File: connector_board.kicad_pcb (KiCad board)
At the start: 2 copper layers, 40 x 22.5 mm, 2 parts, among them J1 Screw Terminal Block 5.00 mm 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

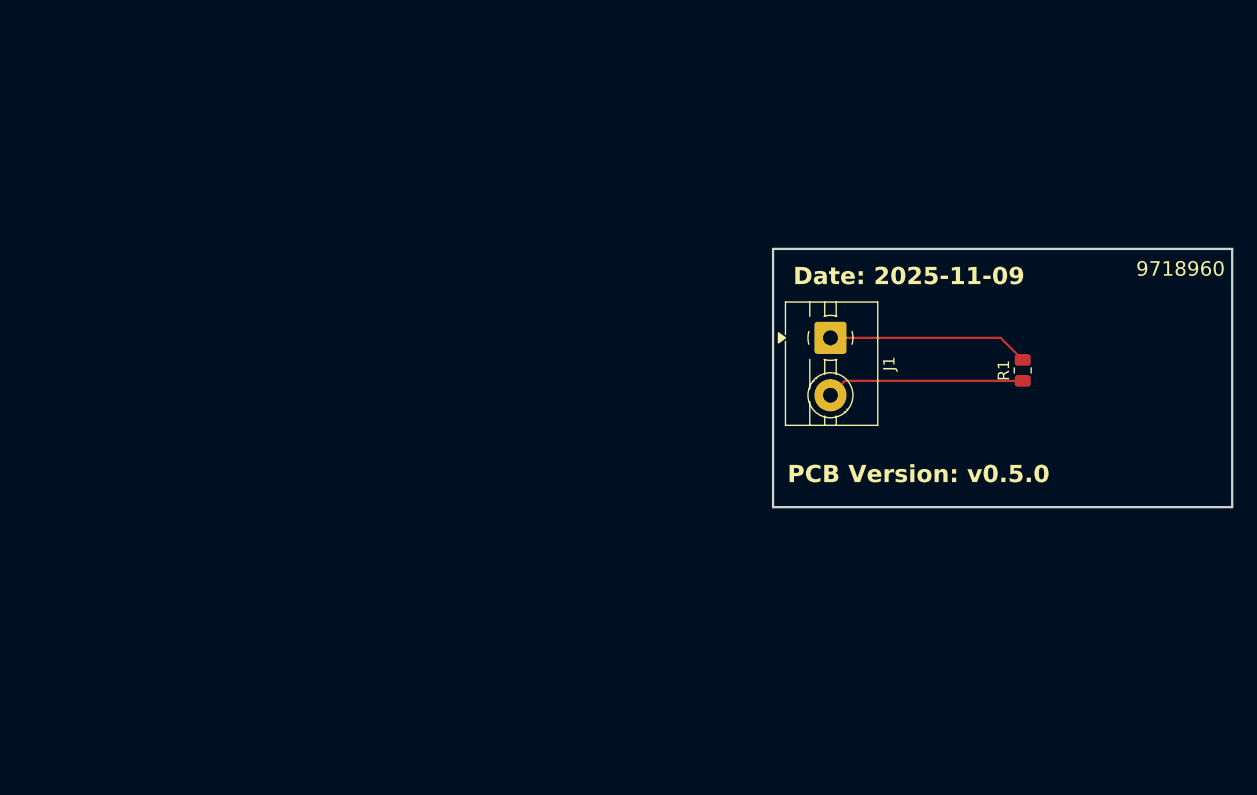
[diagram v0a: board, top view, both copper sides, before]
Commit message: feat: add connectors
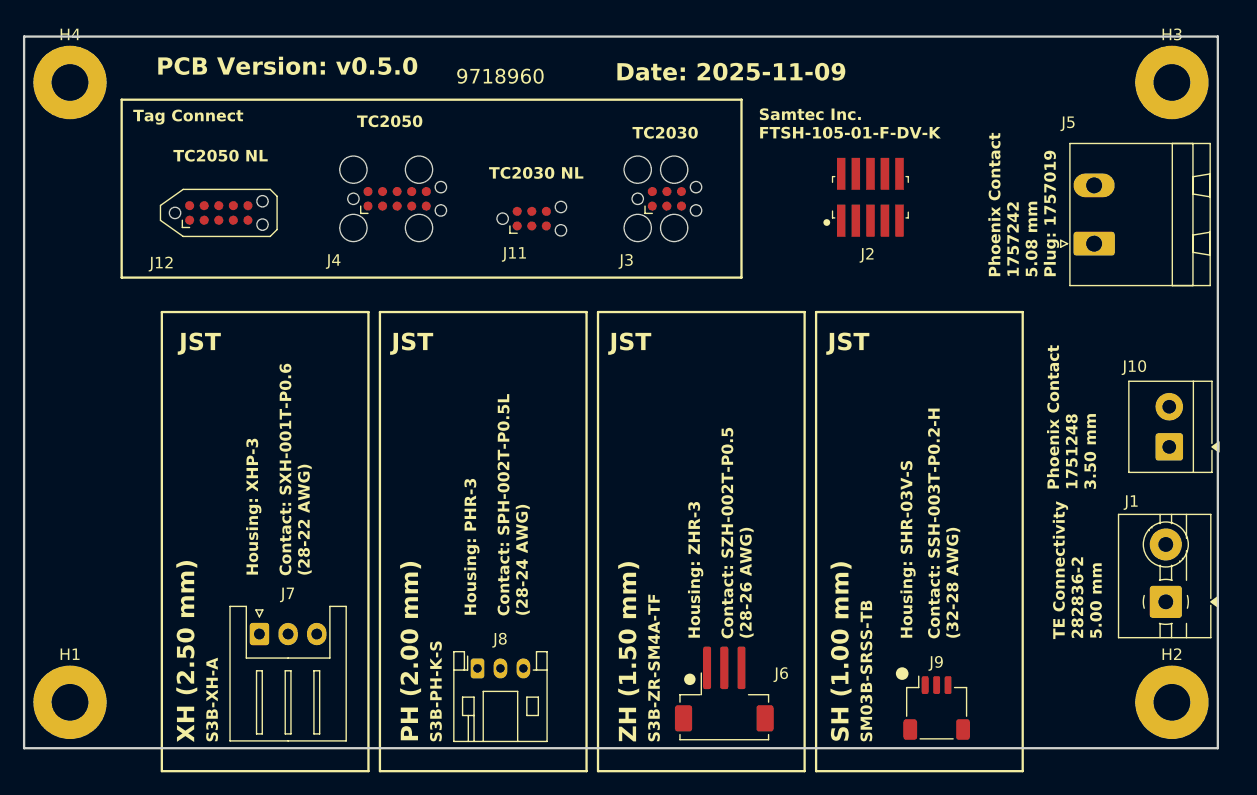
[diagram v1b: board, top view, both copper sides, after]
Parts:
- removed R1: 47k_0805, Resistor_SMD:R_0805_2012Metric
- added H1: MountingHole, MountingHole:MountingHole_3.2mm_M3_Pad, F.Cu at (78.0, 91.0)
- added H2: MountingHole, MountingHole:MountingHole_3.2mm_M3_Pad, F.Cu at (174.0, 91.0)
- added H3: MountingHole, MountingHole:MountingHole_3.2mm_M3_Pad, F.Cu at (174.0, 37.0)
- added H4: MountingHole, MountingHole:MountingHole_3.2mm_M3_Pad, F.Cu at (78.0, 37.0)
- added J10: Screw Terminal Block 3.50 mm 2 pol, 2s_connectors:TerminalBlock_4Ucon_1x02_P3.50mm_Horizontal, F.Cu at (173.8, 68.8)
- added J11: 2s-tc2030-NL, Connector:Tag-Connect_TC2030-IDC-NL_2x03_P1.27mm_Vertical, F.Cu at (118.2, 48.9)
- added J12: TC2050 With UART NL, Connector:Tag-Connect_TC2050-IDC-NL_2x05_P1.27mm_Vertical, F.Cu at (91.0, 48.4)
- added J2: 2s_cortex-m-10-pin, 2s_connectors:PinHeader_2x5_P1.27_SMD, F.Cu at (147.7, 47.0)
- added J3: 2s-tc2030, Connector:Tag-Connect_TC2030-IDC-FP_2x03_P1.27mm_Vertical, F.Cu at (130.0, 47.1)
- added J4: 2s_cortex-m-10-pin, Connector:Tag-Connect_TC2050-IDC-FP_2x05_P1.27mm_Vertical, F.Cu at (106.5, 47.1)
- added J5: 1757242, Connector_Phoenix_MSTB:PhoenixContact_MSTBA_2,5_2-G-5,08_1x02_P5.08mm_Horizontal, F.Cu at (167.2, 51.0)
- added J6: S3B-ZR-SM4A-TF, 2s_connectors:JST_ZH_B3B-ZR-SM4-TF_1x03-1MP_P1.50mm_Vertical, F.Cu at (135.0, 91.0)
- added J7: JST S3B-XH-A, Connector_JST:JST_XH_S3B-XH-A_1x03_P2.50mm_Horizontal, F.Cu at (94.5, 85.1)
- added J8: JST S3B-PH-K-S, Connector_JST:JST_PH_S3B-PH-K_1x03_P2.00mm_Horizontal, F.Cu at (113.5, 88.0)
- added J9: JST SM03B-SRSS-TB, 2s_connectors:JST_SH_SM03B-SRSS-TB_1x03-1MP_P1.00mm_Horizontal, F.Cu at (153.5, 91.5)
- moved J1 37.2 mm to (173.5, 82.2), turned to 90 degrees
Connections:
- J1 pad 1: GND -> unconnected-(J1-Pin_1-Pad1)
- J1 pad 2: Net-(J1-Pin_2) -> unconnected-(J1-Pin_2-Pad2)
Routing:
- net GND: track 17.5 -> 0.00 mm
- net Net-(J1-Pin_2): track 17.3 -> 0.00 mm
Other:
- board size 40 x 22.5 mm -> 104 x 62 mm
- board text added: "Contact: SPH-002T-P0.5L (28-24 AWG)"
- board text added: "Contact: SSH-003T-P0.2-H (32-28 AWG)"
- board text added: "Contact: SXH-001T-P0.6 (28-22 AWG)"
- board text added: "Contact: SZH-002T-P0.5 (28-26 AWG)"
- board text added: "Housing: PHR-3"
- board text added: "Housing: SHR-03V-S"
- board text added: "Housing: XHP-3"
- board text added: "Housing: ZHR-3"
- board text added: "JST"
- board text added: "PH (2.00 mm)"
- board text added: "Phoenix Contact 1751248 3.50 mm"
- board text added: "Phoenix Contact 1757242 5.08 mm Plug: 1757019"
- board text added: "S3B-PH-K-S"
- board text added: "S3B-XH-A"
- board text added: "S3B-ZR-SM4A-TF"
- board text added: "SH (1.00 mm)"
- board text added: "SM03B-SRSS-TB"
- board text added: "Samtec Inc. FTSH-105-01-F-DV-K"
- board text added: "TC2030"
- board text added: "TC2030 NL"
- board text added: "TC2050"
- board text added: "TC2050 NL"
- board text added: "TE Connectivity 282836-2 5.00 mm"
- board text added: "Tag Connect"
- board text added: "XH (2.50 mm)"
- board text added: "ZH (1.50 mm)"
